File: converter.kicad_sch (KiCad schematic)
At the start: 0 parts

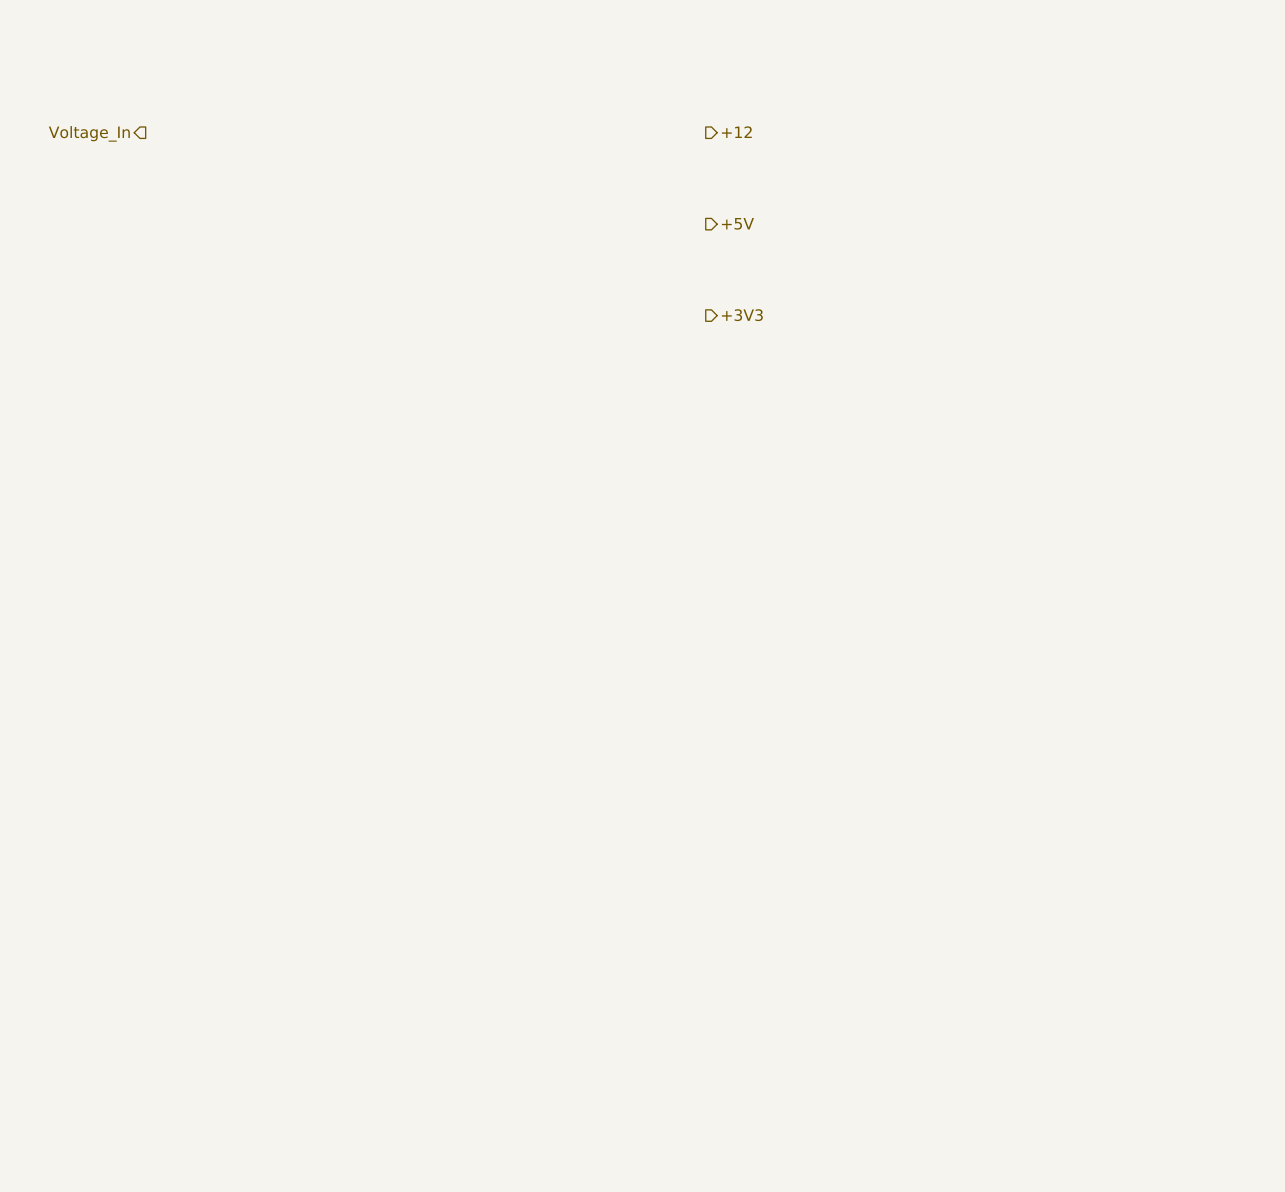
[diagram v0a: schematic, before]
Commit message: lots of lots changes. Schematic done NEEDS Review
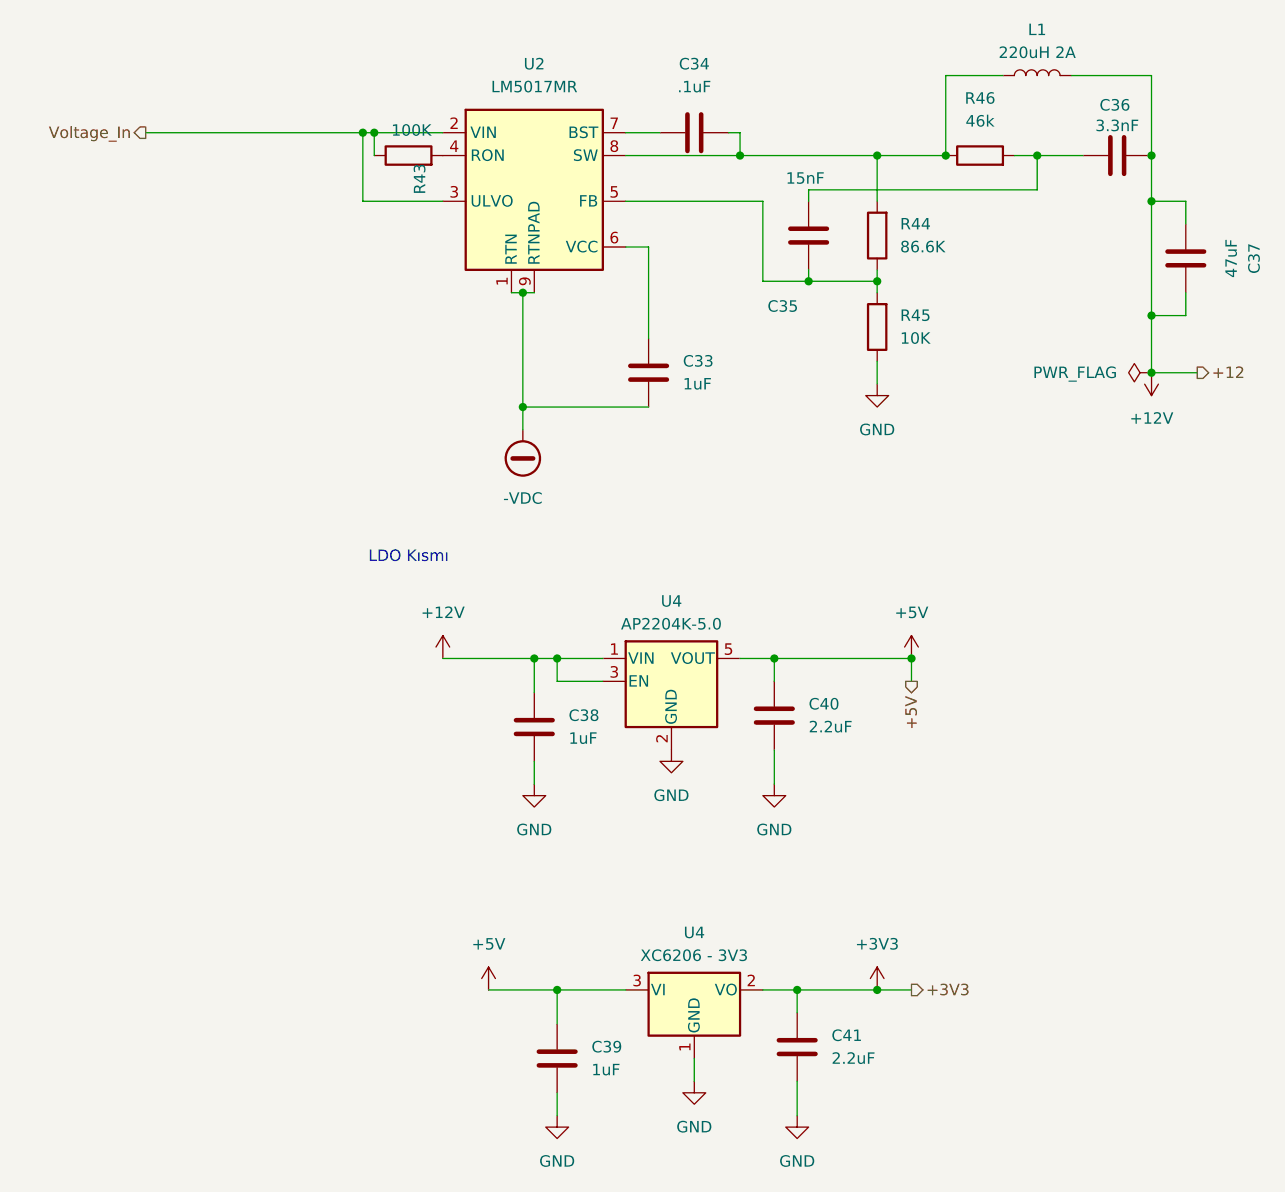
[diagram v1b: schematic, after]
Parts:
- added C33: 1uF, Capacitor_SMD:C_1210_3225Metric_Pad1.33x2.70mm_HandSolder, symbol Device:C
- added C34: .1uF, Capacitor_SMD:C_0603_1608Metric_Pad1.08x0.95mm_HandSolder, symbol Device:C
- added C35: 15nF, Capacitor_SMD:C_0603_1608Metric_Pad1.08x0.95mm_HandSolder, symbol Device:C
- added C36: 3.3nF, Capacitor_SMD:C_0603_1608Metric_Pad1.08x0.95mm_HandSolder, symbol Device:C
- added C37: 47uF, Capacitor_SMD:C_1210_3225Metric_Pad1.33x2.70mm_HandSolder, symbol Device:C
- added C38, C39: 1uF, Capacitor_SMD:C_0603_1608Metric_Pad1.08x0.95mm_HandSolder, symbol Device:C
- added C40, C41: 2.2uF, Capacitor_SMD:C_0603_1608Metric_Pad1.08x0.95mm_HandSolder, symbol Device:C
- added L1: 220uH 2A, Inductor_SMD:L_1210_3225Metric_Pad1.42x2.65mm_HandSolder, symbol Device:L
- added R43: 100K, Resistor_SMD:R_0603_1608Metric_Pad0.98x0.95mm_HandSolder, symbol Device:R
- added R44: 86.6K, Resistor_SMD:R_0603_1608Metric_Pad0.98x0.95mm_HandSolder, symbol Device:R
- added R45: 10K, Resistor_SMD:R_0603_1608Metric_Pad0.98x0.95mm_HandSolder, symbol Device:R
- added R46: 46k, Resistor_SMD:R_0603_1608Metric_Pad0.98x0.95mm_HandSolder, symbol Device:R
- added U2: LM5017MR, Package_SO:SOIC-8-1EP_3.9x4.9mm_P1.27mm_EP2.95x4.9mm_Mask2.71x3.4mm_ThermalVias, symbol Regulator_Switching:LM5017MR
- added U4: AP2204K-5.0, Package_TO_SOT_SMD:SOT-23-5, symbol Regulator_Linear:AP2204K-5.0
- added U4: XC6206 - 3V3, Package_TO_SOT_SMD:SOT-23-3, symbol Regulator_Linear:XC6206PxxxMR
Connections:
- net +3V3: now also C41.1, U4.2 (VO)
- net +5V: now also C39.1, C40.1, U4.3 (VI), U4.5 (VOUT)
- net Voltage_In: now also R43.1, U2.2 (VIN), U2.3 (ULVO)
- new net: C35.1, R44.1, R45.2, U2.5 (FB)
- new net: C35.2, C36.1, R46.2
- new net: C34.1, U2.7 (BST)
- new net: C34.2, L1.1, R44.2, R46.1, U2.8 (SW)
- new net: C33.1, U2.6 (VCC)
- new net: R43.2, U2.4 (RON)
- new net +12V: C36.2, C37.1, C37.2, C38.1, L1.2, U4.1 (VIN), U4.3 (EN)
- new net -VDC: C33.2, U2.1 (RTN), U2.9 (RTNPAD)
- new net GND: C38.2, C39.2, C40.2, C41.2, R45.1, U4.1 (GND), U4.2 (GND)
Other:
- note added: "LDO Kısmı"
- company: (none) -> Pehlivan Team
- title: (none) -> Pehli-Shell-BMS
